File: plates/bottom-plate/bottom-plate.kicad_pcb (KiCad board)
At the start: 2 copper layers, 140.5 x 112.5 mm, 0 parts

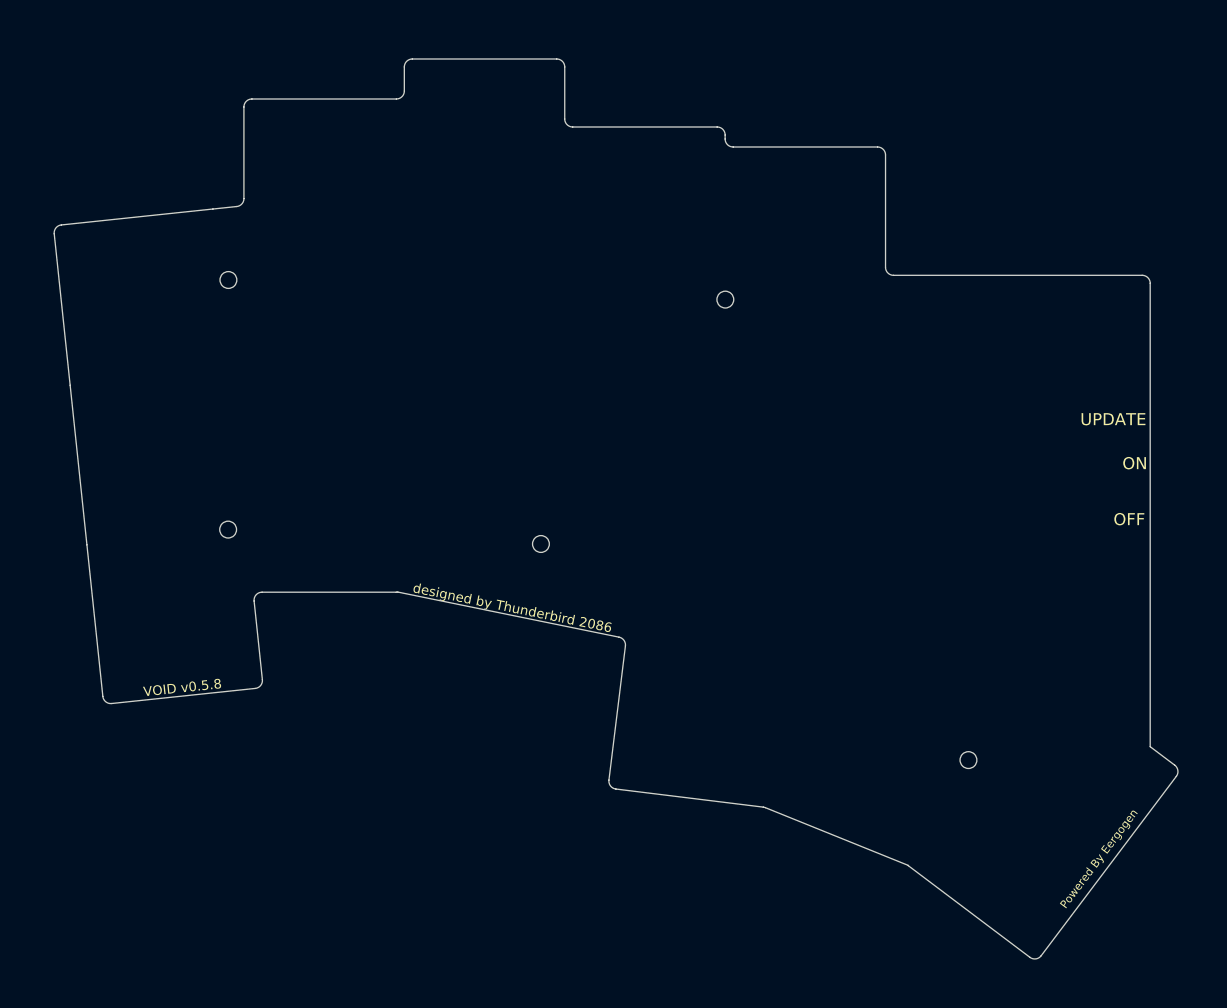
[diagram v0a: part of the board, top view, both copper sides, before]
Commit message: added hybrid
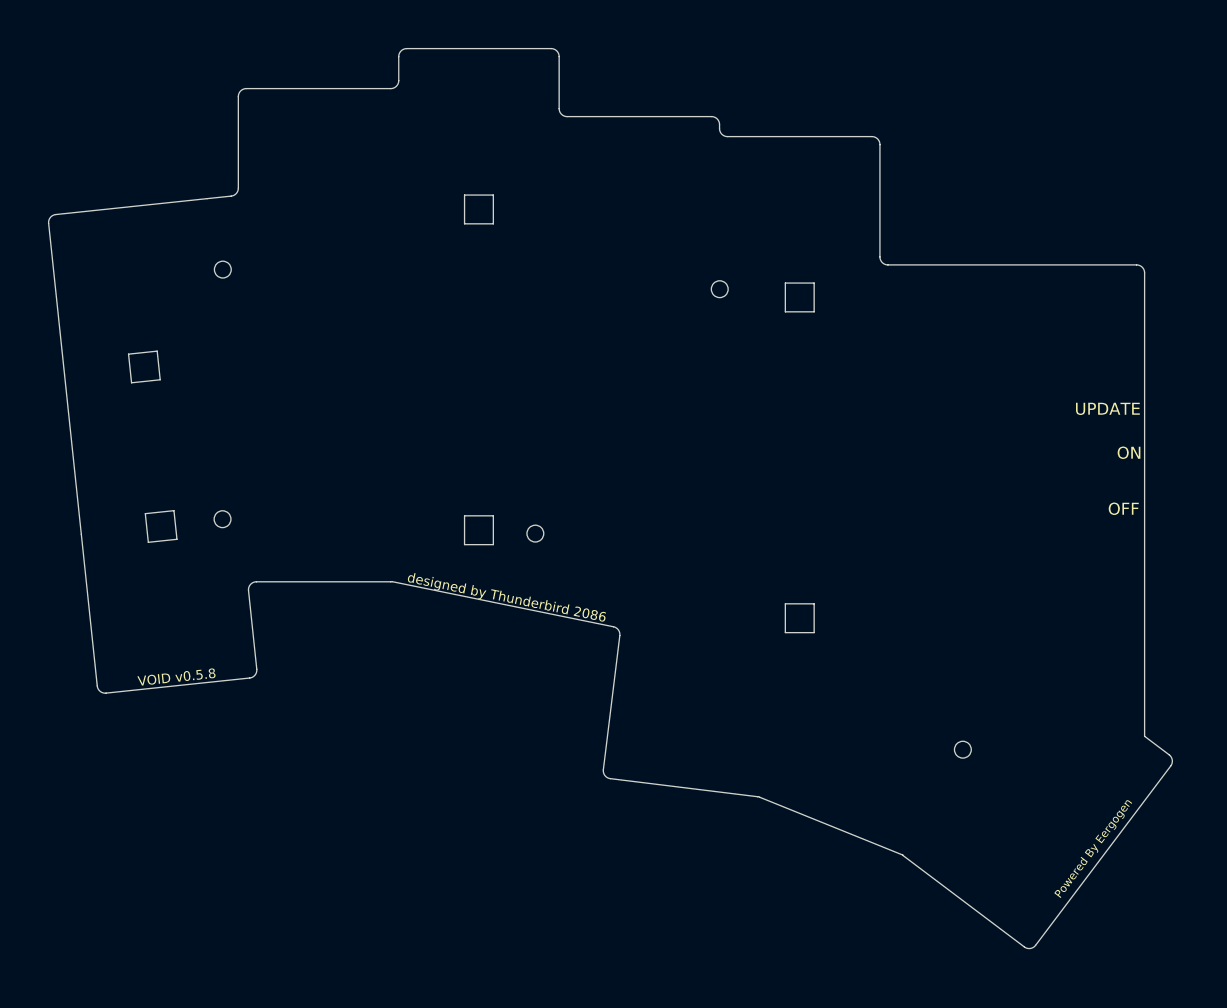
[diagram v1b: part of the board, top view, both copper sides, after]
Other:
- outline, holes or cut-outs redrawn
